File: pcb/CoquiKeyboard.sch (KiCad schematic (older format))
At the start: 116 parts

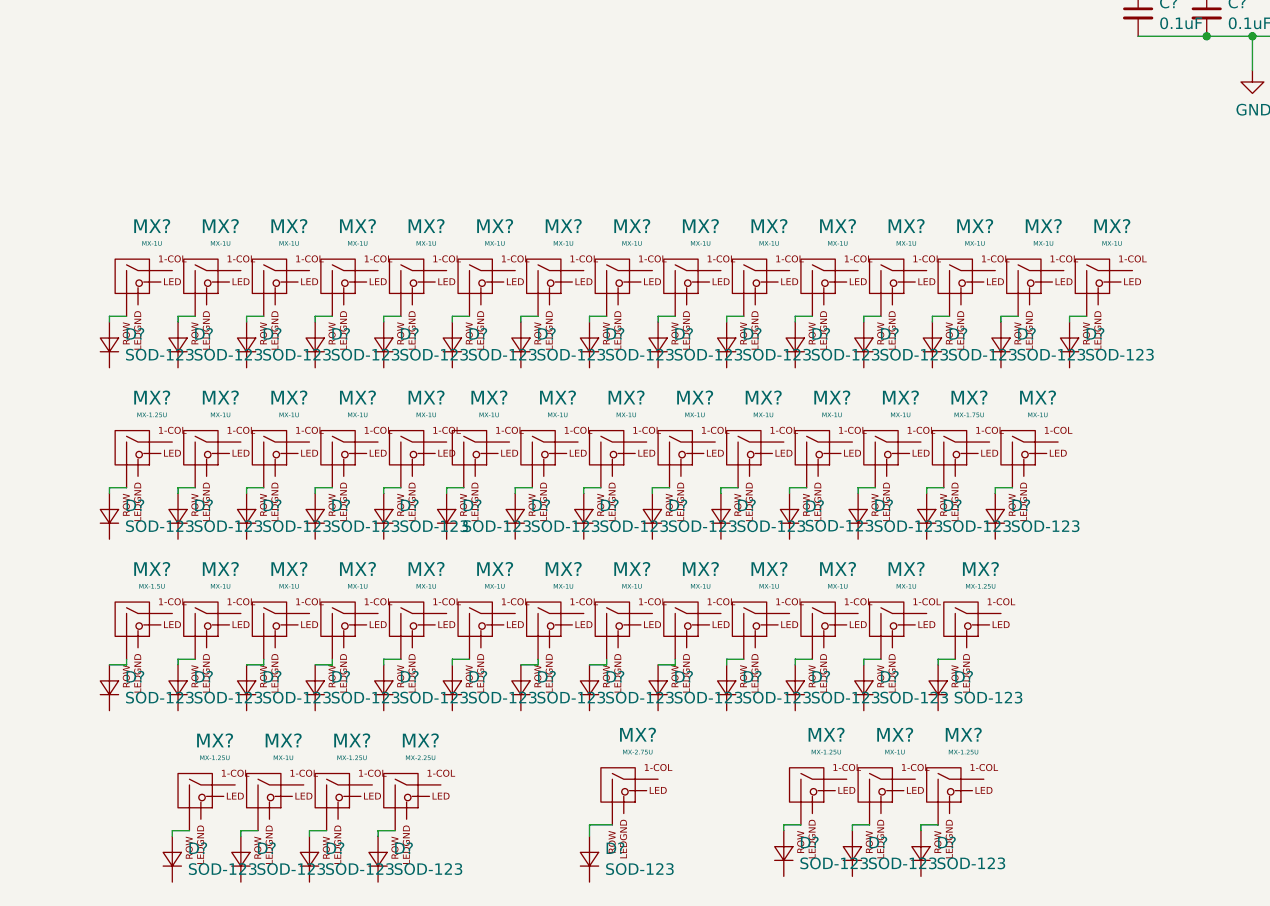
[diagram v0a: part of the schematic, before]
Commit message: draw matrices
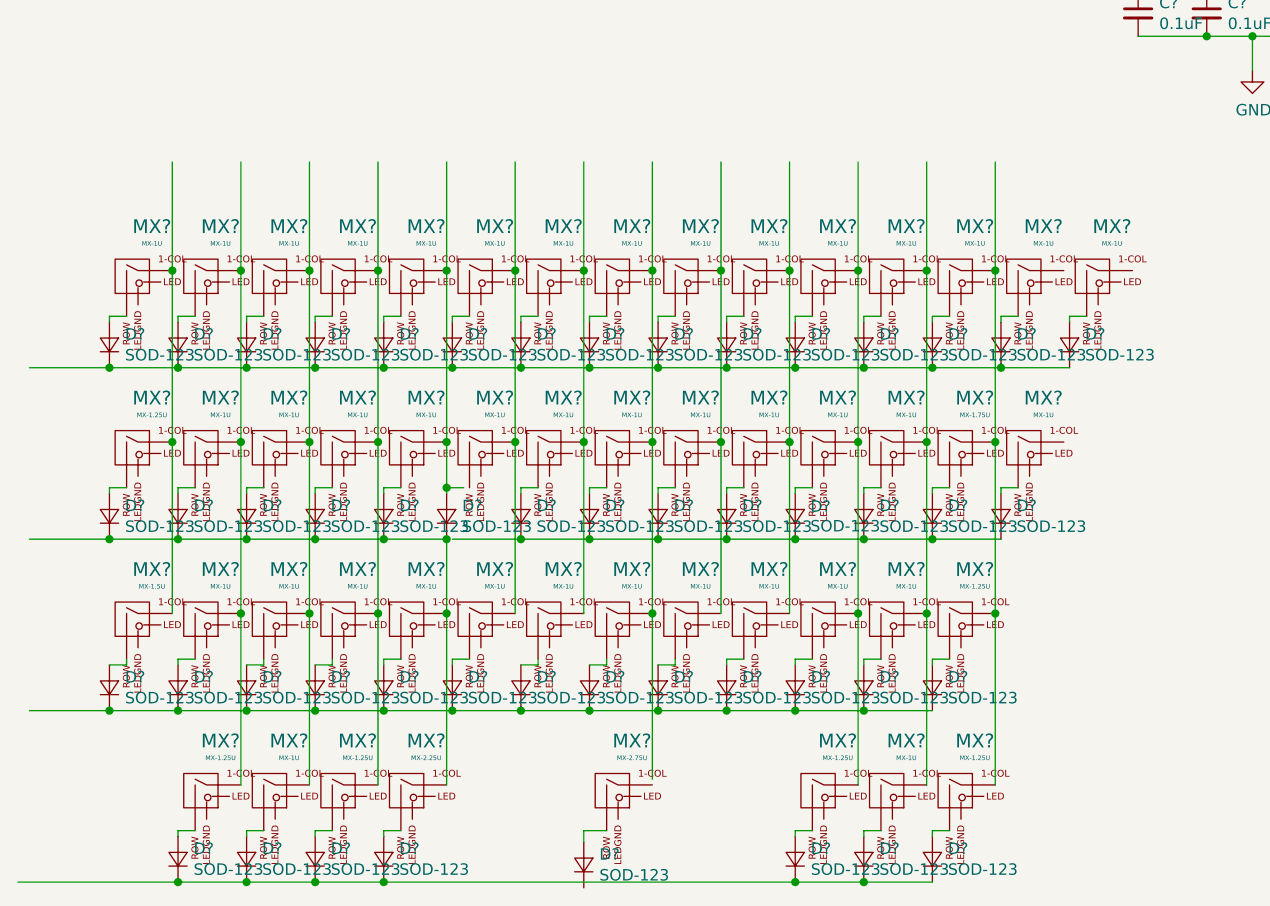
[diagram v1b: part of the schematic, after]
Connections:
- wire segments 149 -> 246
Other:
- moved on the sheet: D?, MX?
